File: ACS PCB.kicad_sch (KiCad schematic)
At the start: 1 part

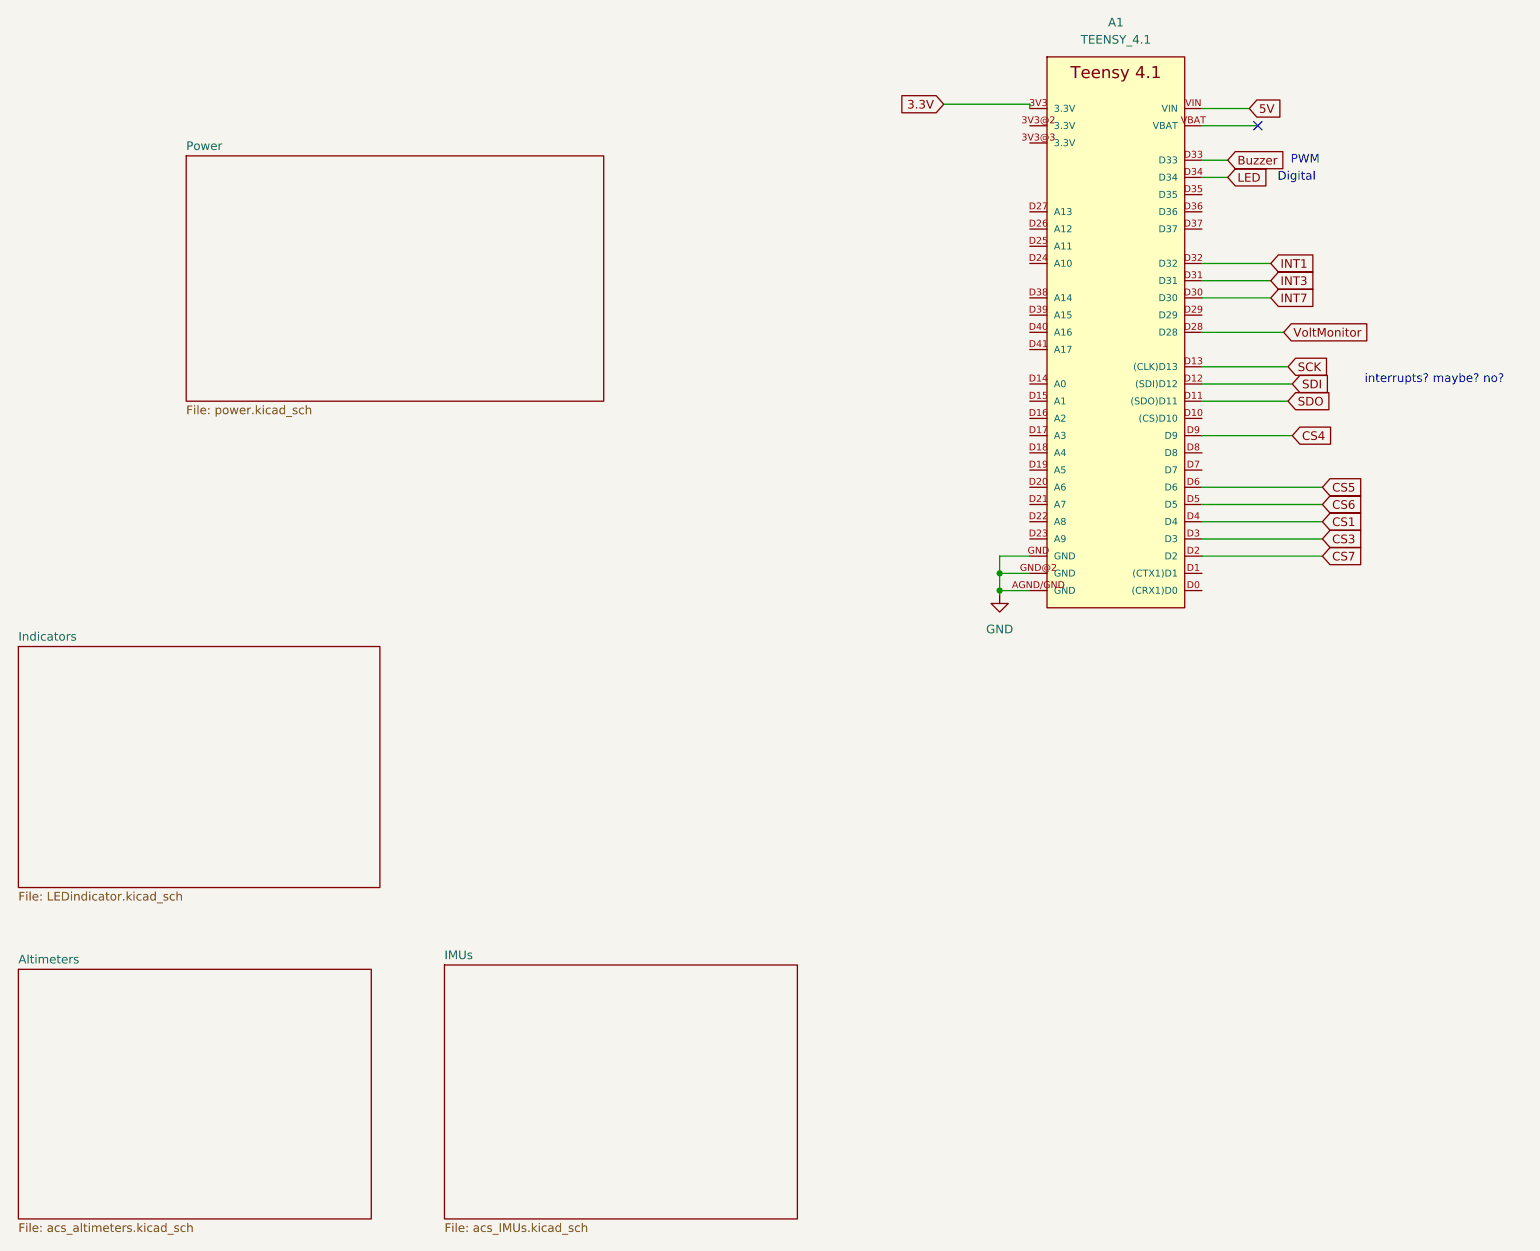
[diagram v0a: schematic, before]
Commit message: Fixed symbols and ran ERC
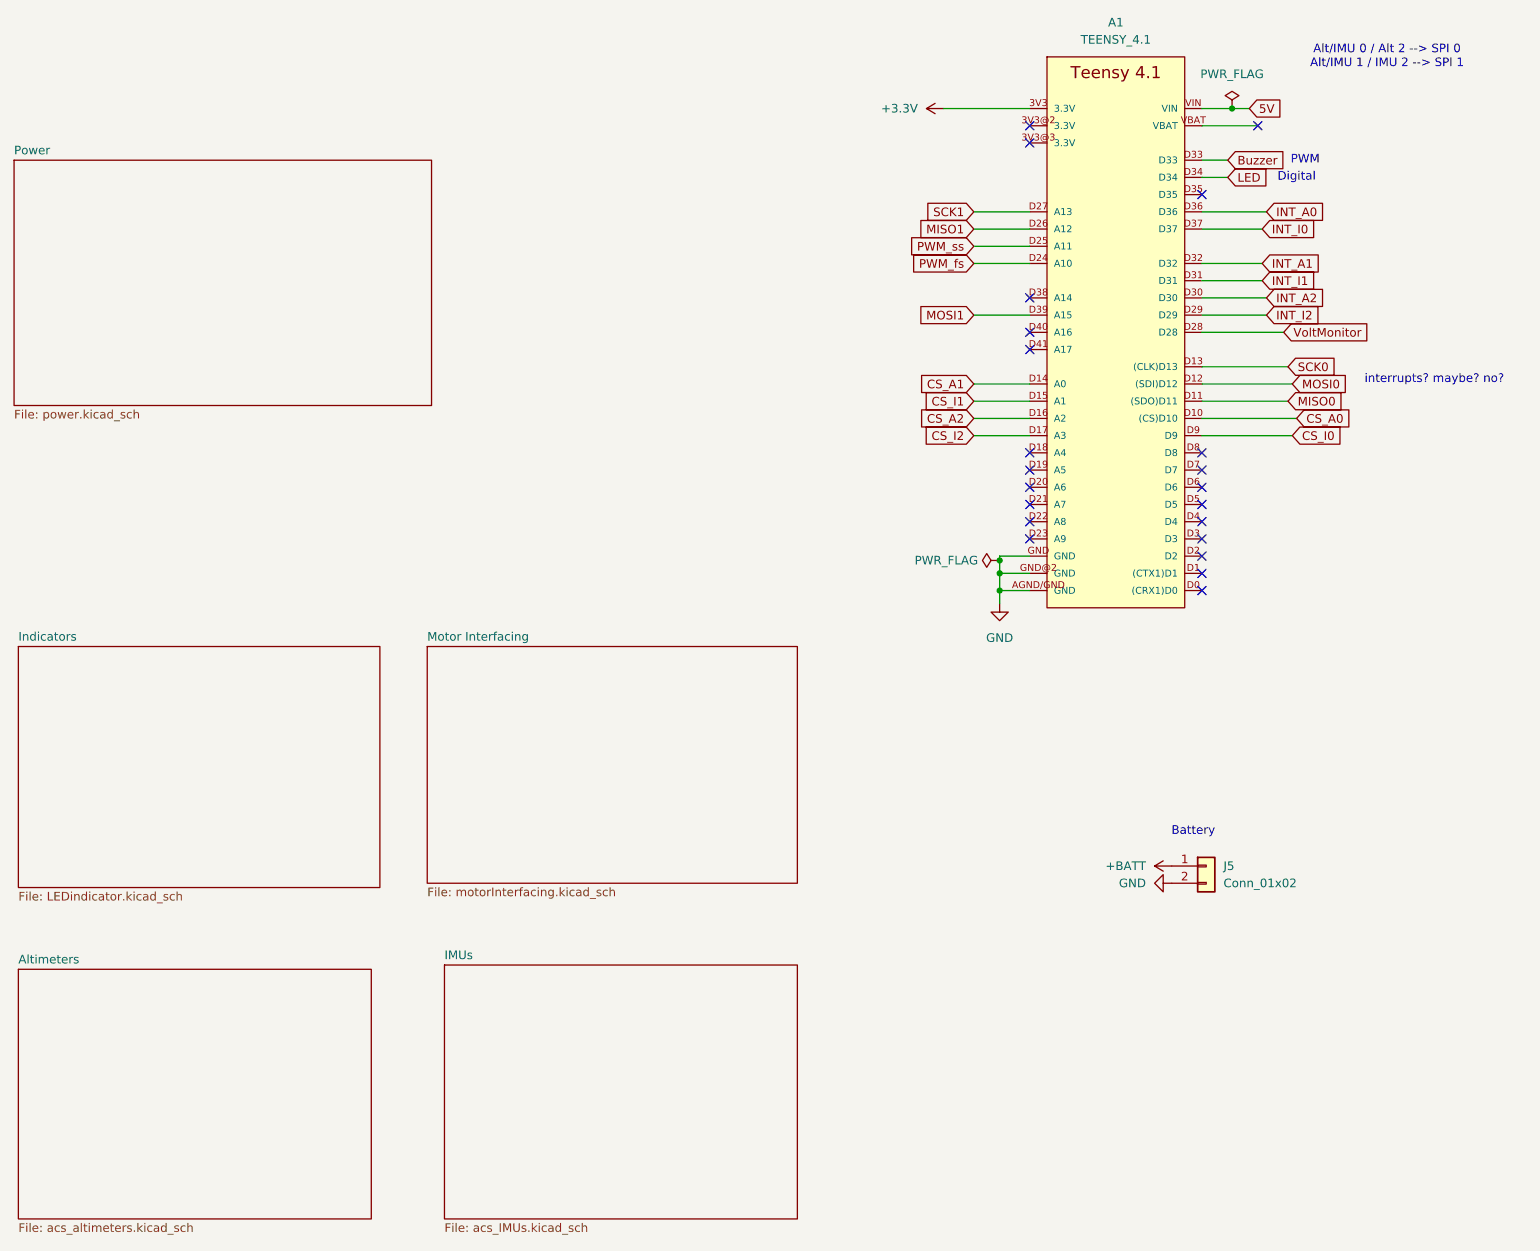
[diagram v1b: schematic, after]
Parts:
- added J5: Conn_01x02, symbol Connector_Generic:Conn_01x02
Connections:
- net GND: now also J5.2 (Pin_2)
- net CS_A0: now reaches A1.D10 ((CS)D10)
- net CS_A1: now reaches A1.D14 (A0)
- net CS_I1: now reaches A1.D15 (A1)
- net CS_A2: now reaches A1.D16 (A2)
- net CS_I2: now reaches A1.D17 (A3)
- net PWM_fs: now reaches A1.D24 (A10)
- net PWM_ss: now reaches A1.D25 (A11)
- net MISO1: now reaches A1.D26 (A12)
- net SCK1: now reaches A1.D27 (A13)
- net INT_I2: now reaches A1.D29
- net INT_A0: now reaches A1.D36
- net INT_I0: now reaches A1.D37
- net MOSI1: now reaches A1.D39 (A15)
- net 3.3V renamed +3.3V
- net CS1: no longer names the net of A1.D4
- net CS3: no longer names the net of A1.D3
- net CS4 renamed CS_I0
- net CS5: no longer names the net of A1.D6
- net CS6: no longer names the net of A1.D5
- net CS7: no longer names the net of A1.D2
- net INT1 renamed INT_A1
- net INT3 renamed INT_I1
- net INT7 renamed INT_A2
- net SCK renamed SCK0
- net SDI renamed MOSI0
- net SDO renamed MISO0
- new net +BATT: J5.1 (Pin_1)
- no-connect marks 1 -> 22
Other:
- added sheet Motor Interfacing (motorInterfacing.kicad_sch)
- note added: "Alt/IMU 0 / Alt 2 --> SPI 0 Alt/IMU 1 / IMU 2 --> SPI 1"
- note added: "Battery"

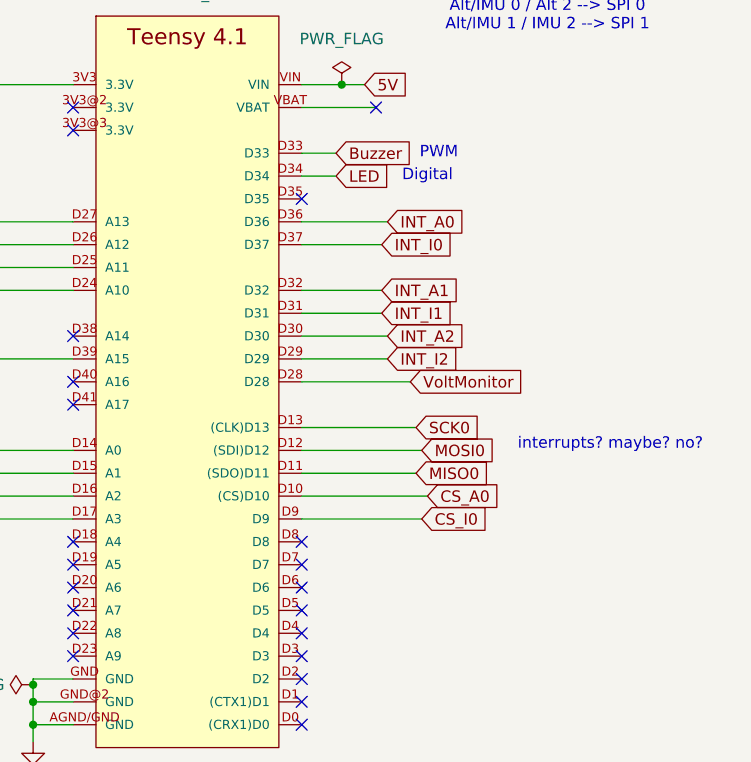
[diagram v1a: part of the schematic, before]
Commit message: added-more-leds
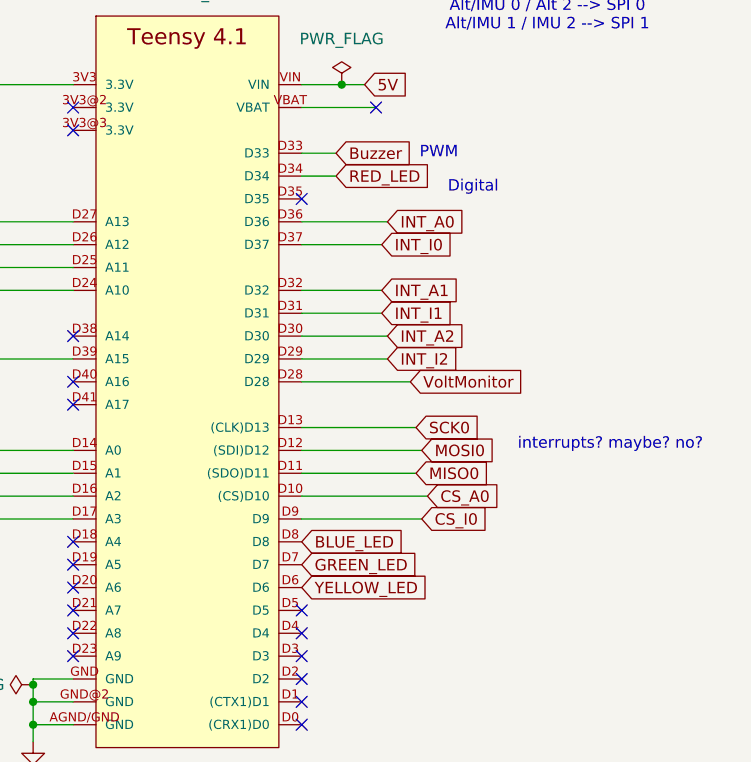
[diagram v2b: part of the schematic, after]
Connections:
- net YELLOW_LED: now reaches A1.D6
- net GREEN_LED: now reaches A1.D7
- net BLUE_LED: now reaches A1.D8
- net LED renamed RED_LED
- no-connect marks 22 -> 19
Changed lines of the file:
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@@
 	(text "Digital"
 		(exclude_from_sim no)
-		(at 226.06 43.18 0)
+		(at 231.14 44.45 0)
 		(effects
 			(font
@@
 	)
 	(no_connect
-		(at 212.09 88.9)
-	)
-	(no_connect
 		(at 212.09 93.98)
 	)
@@
 	)
 	(no_connect
-		(at 212.09 86.36)
-	)
-	(no_connect
 		(at 186.69 96.52)
 	)
@@
 	)
 	(no_connect
-		(at 212.09 83.82)
-	)
-	(no_connect
 		(at 186.69 38.1)
 	)
@@
 		)
 	)
+	(global_label "BLUE_LED"
+		(shape input)
+		(at 212.09 83.82 0)
+		(fields_autoplaced yes)
+		(effects
+			(font
+				(size 1.27 1.27)
+			)
+			(justify left)
+		)
+		(property "Intersheetrefs" "${INTERSHEET_REFS}"
+			(at 224.2675 83.82 0)
+			(hide yes)
+			(show_name no)
+			(do_not_autoplace no)
+			(effects
+				(font
+					(size 1.27 1.27)
+				)
+				(justify left)
+			)
+		)
+	)
 	(global_label "SCK1"
 		(shape input)
@@
 		)
 	)
-	(global_label "LED"
+	(global_label "RED_LED"
 		(shape input)
 		(at 215.9 43.18 0)
@@
 		)
 		(property "Intersheetrefs" "${INTERSHEET_REFS}"
-			(at 222.3323 43.18 0)
+			(at 226.9889 43.18 0)
 			(hide yes)
 			(show_name no)
@@
 		)
 	)
+	(global_label "GREEN_LED"
+		(shape input)
+		(at 212.09 86.36 0)
+		(fields_autoplaced yes)
+		(effects
+			(font
+				(size 1.27 1.27)
+			)
+			(justify left)
+		)
+		(property "Intersheetrefs" "${INTERSHEET_REFS}"
+			(at 225.6584 86.36 0)
+			(hide yes)
+			(show_name no)
+			(do_not_autoplace no)
+			(effects
+				(font
+					(size 1.27 1.27)
+				)
+				(justify left)
+			)
+		)
+	)
 	(global_label "INT_I0"
 		(shape input)
@@
 			(hide yes)
 			(show_name no)
+			(do_not_autoplace no)
+			(effects
+				(font
+					(size 1.27 1.27)
+				)
+				(justify left)
+			)
+		)
+	)
+	(global_label "YELLOW_LED"
+		(shape input)
+		(at 212.09 88.9 0)
+		(fields_autoplaced yes)
+		(effects
+			(font
+				(size 1.27 1.27)
+			)
+			(justify left)
+		)
+		(property "Intersheetrefs" "${INTERSHEET_REFS}"
+			(at 226.5656 88.9 0)
+			(hide yes)
+			(show_name no)
